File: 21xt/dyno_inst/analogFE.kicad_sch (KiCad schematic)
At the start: 74 parts, among them U12 1SS362FV_L3F, U13 1SS362FV_L3F, U14 ADA4807-2ARM, U15 ADA4807-2ARM, U16 ADA4945-1ACPZ-R2, U17 1SS362FV_L3F, U18 1SS362FV_L3F, U19 ADA4807-1, U20 ADA4807-1, U21 1SS362FV_L3F, U22 ADA4945-1ACPZ-R2

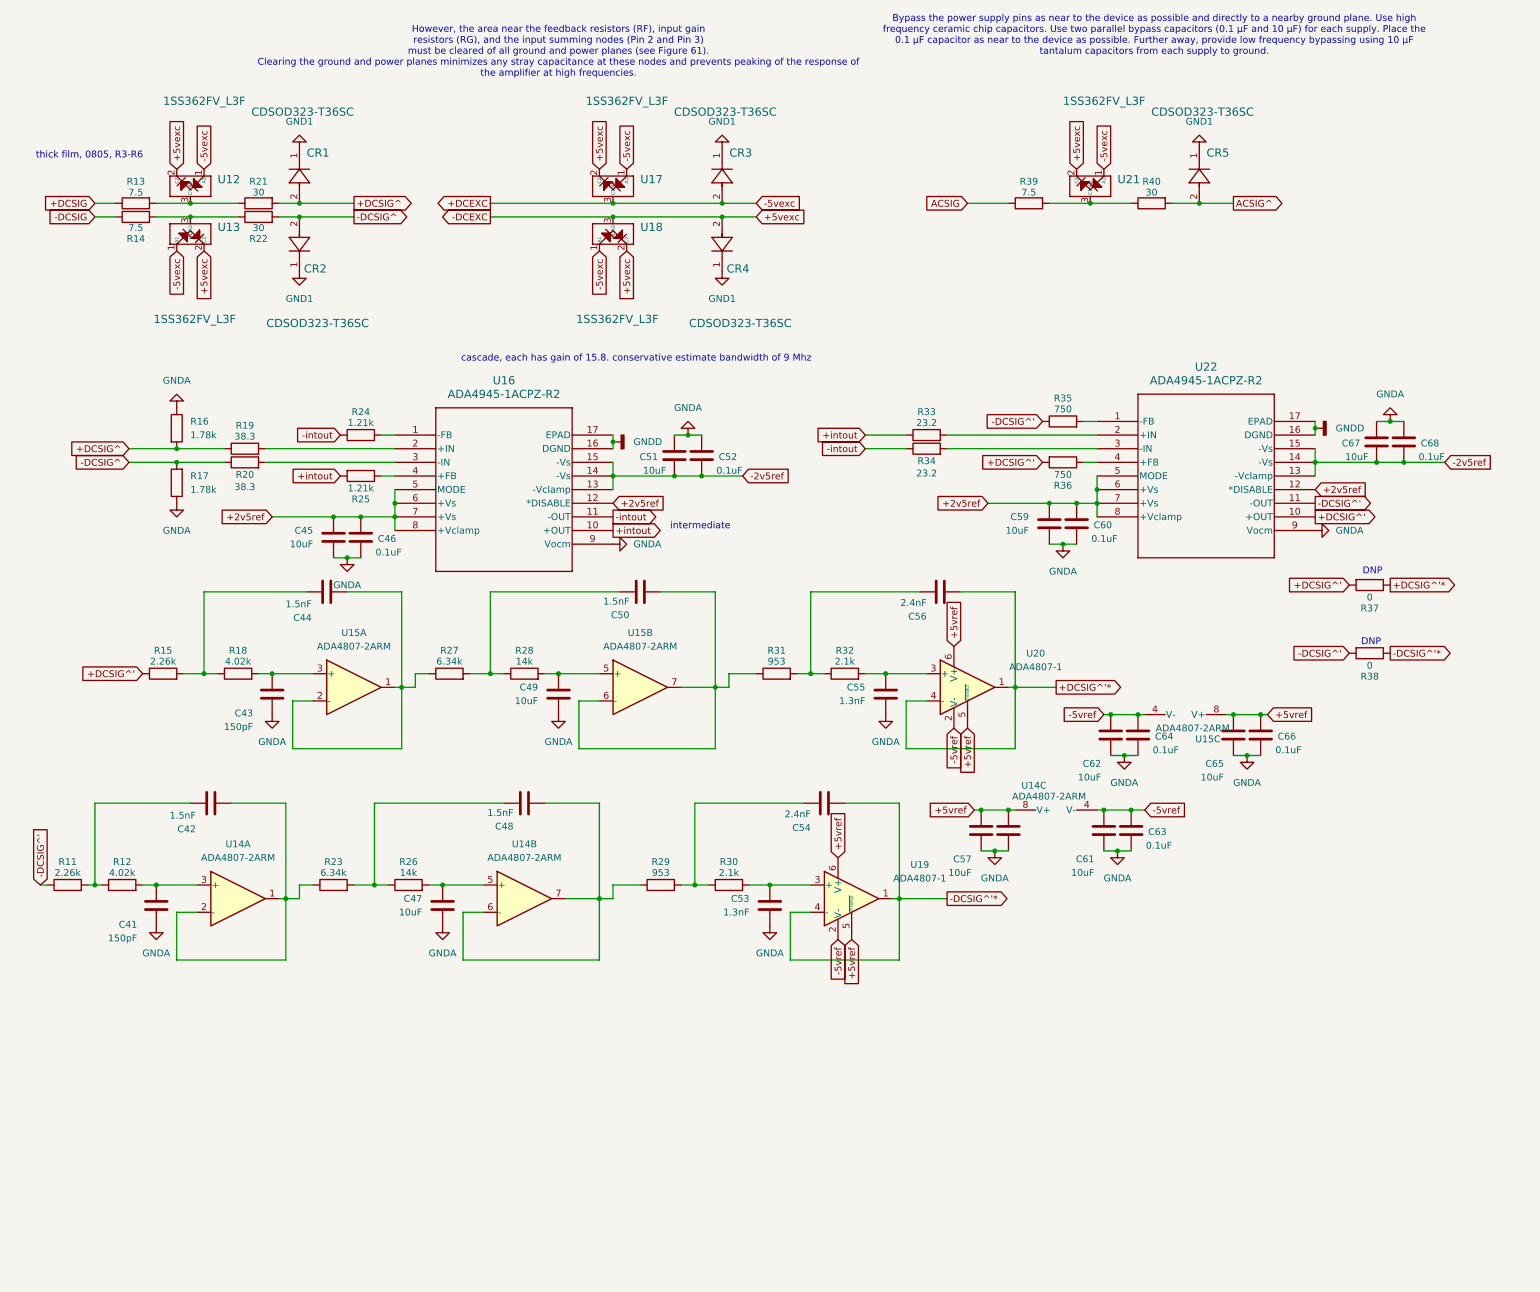
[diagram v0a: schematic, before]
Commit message: adasd
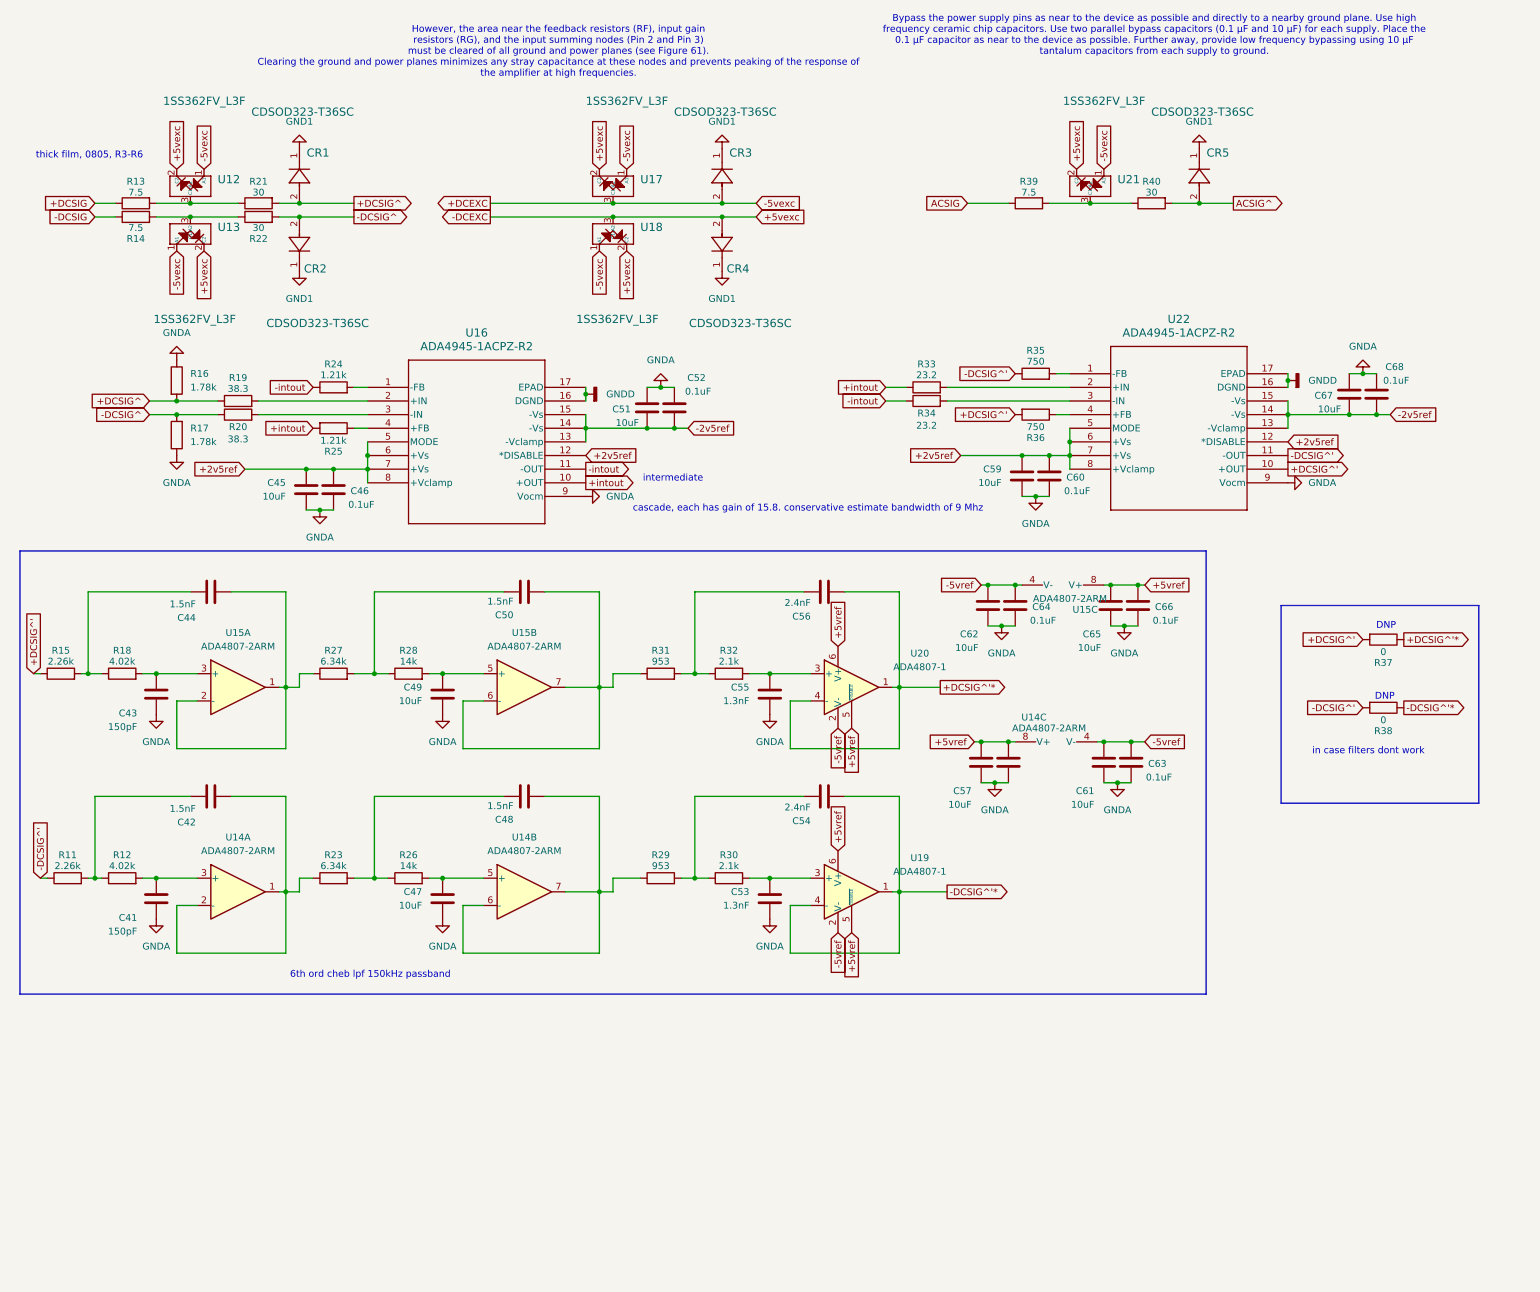
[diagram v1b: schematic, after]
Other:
- note added: "6th ord cheb lpf 150kHz passband"
- note added: "in case filters dont work"
- moved on the sheet: C41, C42, C43, C44, C45, C46, C47, C48, C49, C50, C51, C52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

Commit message: sss
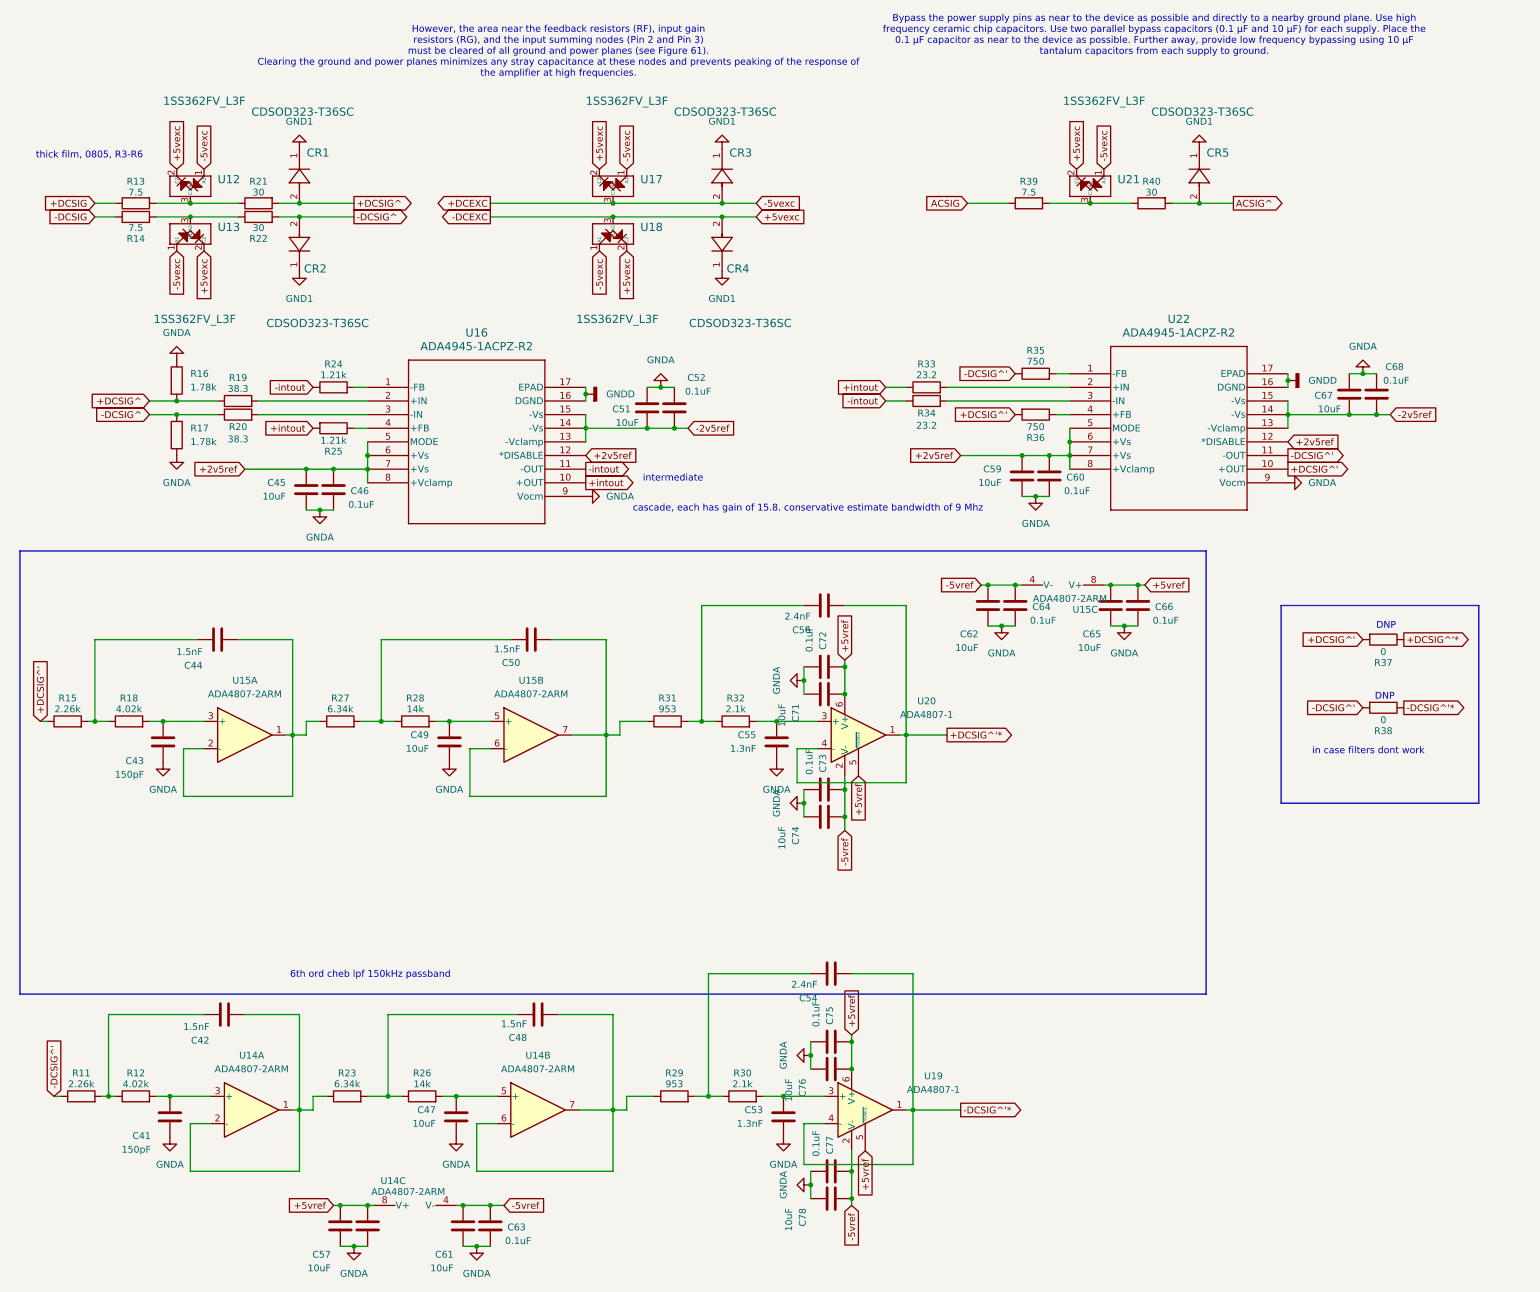
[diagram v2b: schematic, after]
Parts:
- added C71, C74, C76, C78: 10uF, Capacitor_SMD:C_0402_1005Metric, symbol Device:C
- added C72, C73, C75, C77: 0.1uF, Capacitor_SMD:C_0402_1005Metric, symbol Device:C
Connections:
- net +5vref: now also C71.1, C72.1, C75.1, C76.1
- net -5vref: now also C73.1, C74.1, C77.1, C78.1
- net GNDA: now also C71.2, C72.2, C73.2, C74.2, C75.2, C76.2, C77.2, C78.2
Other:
- moved on the sheet: C41, C42, C43, C44, C47, C48, C49, C50, C53, C54, C55, C56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
